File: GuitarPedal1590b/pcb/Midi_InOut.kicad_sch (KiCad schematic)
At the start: 7 parts, among them U5 H11L1

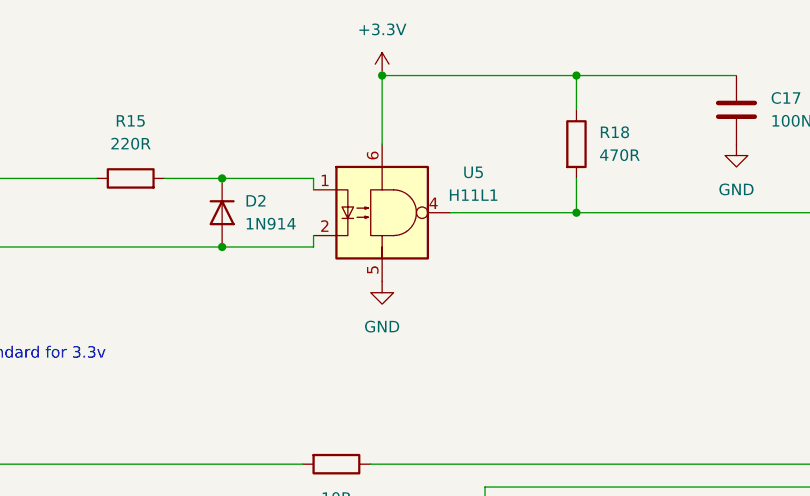
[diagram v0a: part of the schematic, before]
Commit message: Updated project to KiCad 7
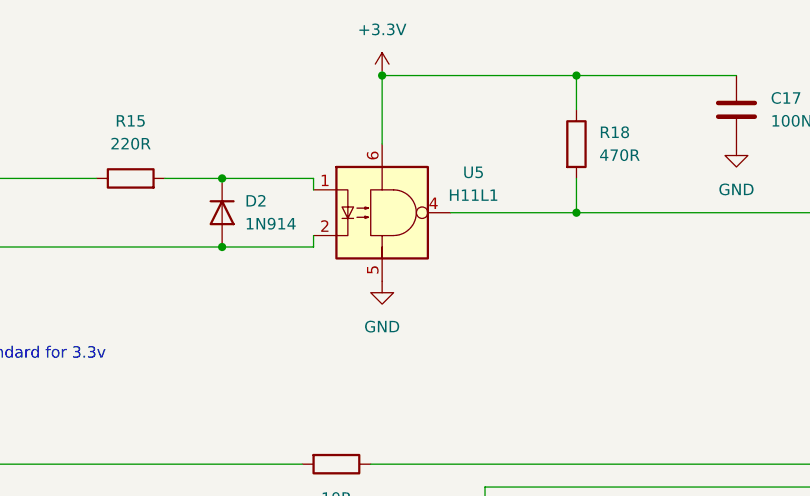
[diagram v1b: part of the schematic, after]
